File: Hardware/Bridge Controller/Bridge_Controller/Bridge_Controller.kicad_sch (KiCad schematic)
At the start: 2 parts, among them J2 AVR-UPDI-6, U2 AVR128DA64x-xPT

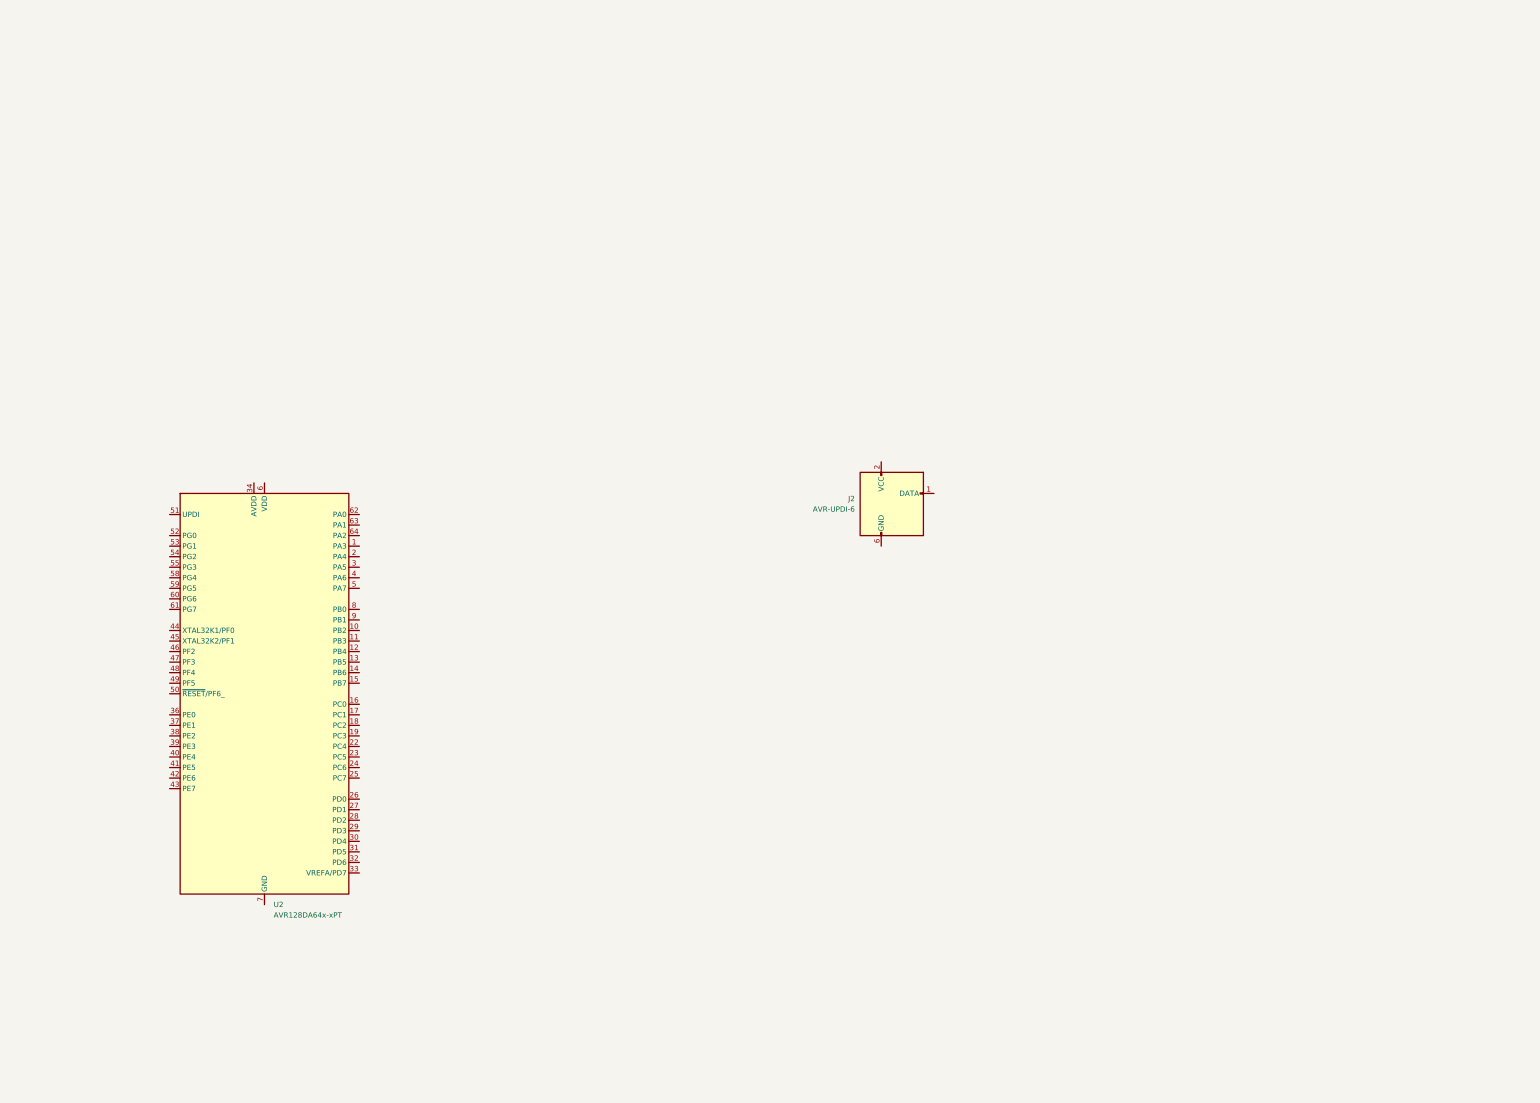
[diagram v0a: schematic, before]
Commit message: Updates to Bridge controller
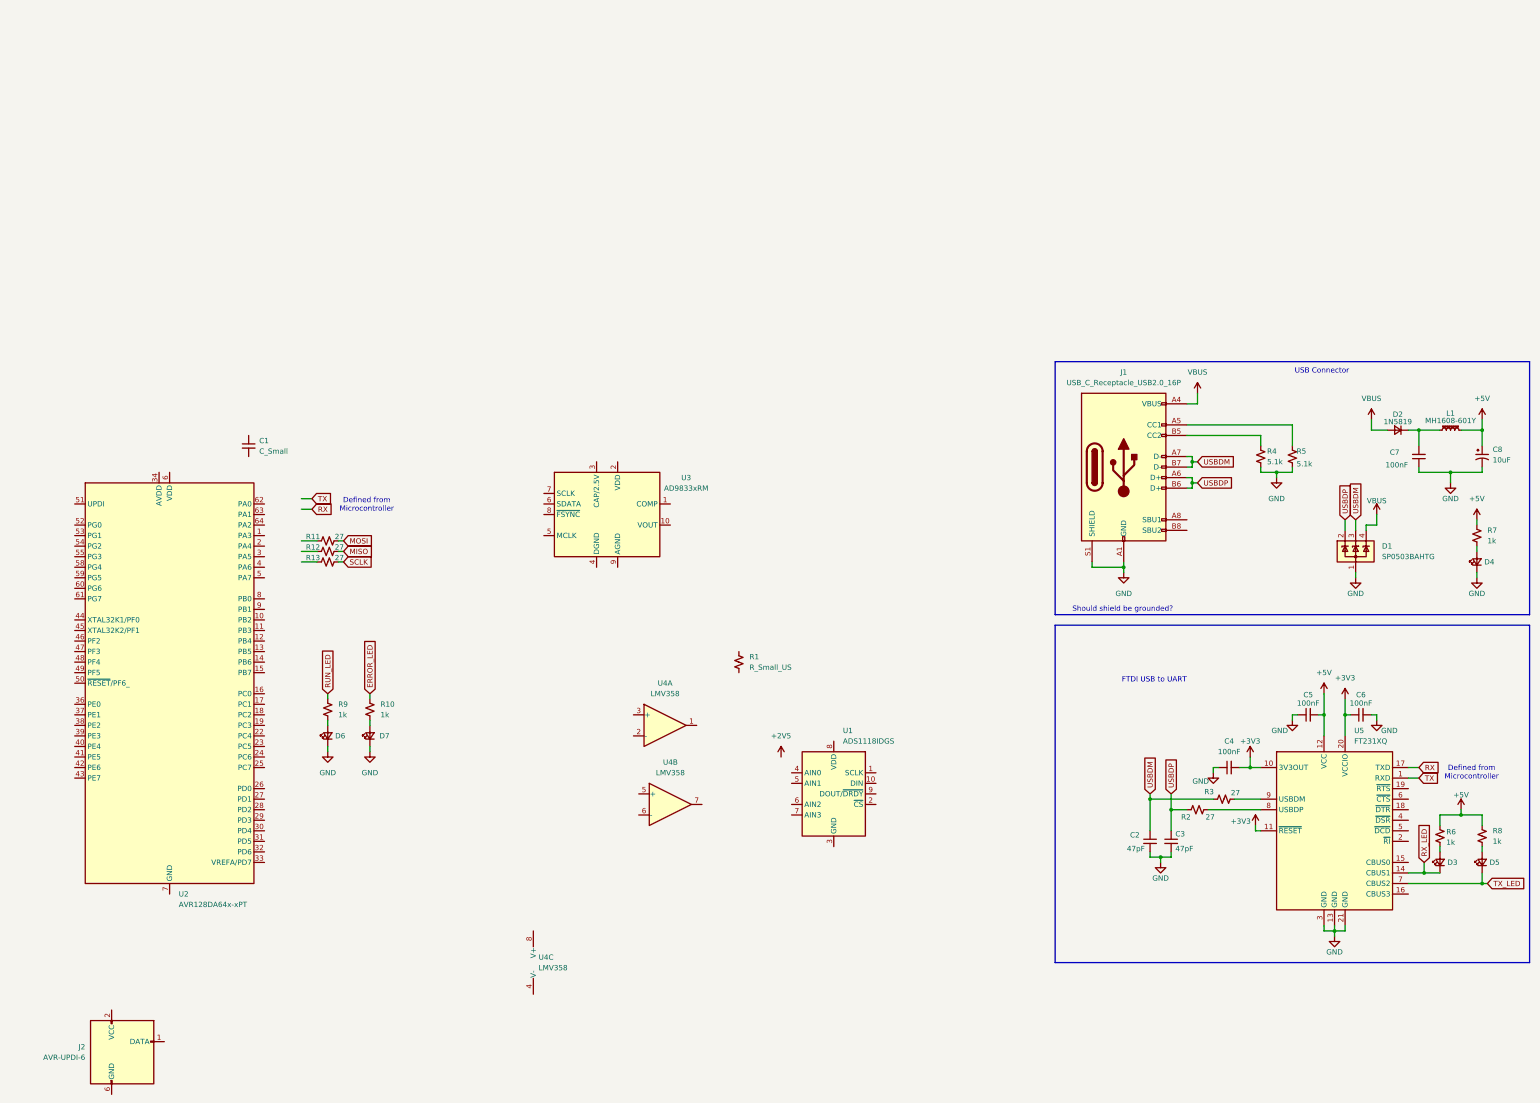
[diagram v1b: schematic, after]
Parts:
- added C1: C_Small, symbol Device:C_Small
- added C2, C3: 47pF, Capacitor_SMD:C_0402_1005Metric, symbol Device:C_Small
- added C4, C5, C6, C7: 100nF, Capacitor_SMD:C_0402_1005Metric, symbol Device:C_Small
- added C8: 10uF, Capacitor_Tantalum_SMD:CP_EIA-3216-18_Kemet-A, symbol Device:C_Polarized_Small_US
- added D1: SP0503BAHTG, Package_TO_SOT_SMD:SOT-143, symbol Power_Protection:SP0503BAHT
- added D2: 1N5819, Diode_SMD:D_SOD-123, symbol Device:D_Small
- added D3, D4, D5, D6: 150080VS75000, LED_SMD:LED_0805_2012Metric, symbol Device:LED_Small
- added D7: 150080SS75000, LED_SMD:LED_0805_2012Metric, symbol Device:LED_Small
- added J1: USB_C_Receptacle_USB2.0_16P, Connector_USB:USB_C_Receptacle_GCT_USB4085, symbol Connector:USB_C_Receptacle_USB2.0_16P
- added L1: MH1608-601Y, Inductor_SMD:L_0603_1608Metric, symbol Device:L_Ferrite_Small
- added R1: R_Small_US, symbol Device:R_Small_US
- added R10, R6, R7, R8, R9: 1k, Resistor_SMD:R_0603_1608Metric, symbol Device:R_Small_US
- added R11, R12, R13, R2, R3: 27, Resistor_SMD:R_0603_1608Metric, symbol Device:R_Small_US
- added R4, R5: 5.1k, Resistor_SMD:R_0603_1608Metric, symbol Device:R_Small_US
- added U1: ADS1118IDGS, symbol Analog_ADC:ADS1118IDGS
- added U3: AD9833xRM, Package_SO:MSOP-10_3x3mm_P0.5mm, symbol Interface:AD9833xRM
- added U4: LMV358, symbol Amplifier_Operational:LMV358
- added U5: FT231XQ, Package_DFN_QFN:QFN-20-1EP_4x4mm_P0.5mm_EP2.5x2.5mm, symbol Interface_USB:FT231XQ
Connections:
- new net: C7.2, D2.1 (K), L1.1
- new net: R2.2, U5.8 (USBDP)
- new net: R3.2, U5.9 (USBDM)
- new net: D3.2 (A), R6.2
- new net: D5.2 (A), R8.2
- new net: J1.A5 (CC1), R5.1
- new net: J1.B5 (CC2), R4.1
- new net: D4.2 (A), R7.2
- new net: D6.2 (A), R9.2
- new net: D7.2 (A), R10.2
- new net +3V3: C4.2, C6.1, U5.10 (3V3OUT), U5.11 (~{RESET}), U5.20 (VCCIO)
- new net +5V: C5.2, C8.1, L1.2, R6.1, R7.1, R8.1, U5.12 (VCC)
- new net ERROR_LED: R10.1
- new net GND: C2.2, C3.2, C4.1, C5.1, C6.2, C7.1, C8.2, D1.1 (A), D4.1 (K), D6.1 (K), D7.1 (K), J1.A1 (GND), J1.A12 (GND), J1.B1 (GND), J1.B12 (GND), J1.S1 (SHIELD), R4.2, R5.2, U5.13 (GND), U5.21 (GND), U5.3 (GND)
- new net MISO: R12.2
- new net MOSI: R11.2
- new net RUN_LED: R9.1
- new net RX: U5.17 (TXD)
- new net RX_LED: D3.1 (K), U5.14 (CBUS1)
- new net SCLK: R13.2
- new net TX: U5.1 (RXD)
- new net TX_LED: D5.1 (K), U5.7 (CBUS2)
- new net USBDM: C2.1, D1.3 (K), J1.A7 (D-), J1.B7 (D-), R3.1
- new net USBDP: C3.1, D1.2 (K), J1.A6 (D+), J1.B6 (D+), R2.1
- new net VBUS: D1.4 (K), D2.2 (A), J1.A4 (VBUS), J1.A9 (VBUS), J1.B4 (VBUS), J1.B9 (VBUS)
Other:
- note added: "Defined from Microcontroller"
- note added: "FTDI USB to UART"
- note added: "Should shield be grounded?"
- note added: "USB Connector"
- moved on the sheet: J2, U2

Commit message: Updating Bridge Controller
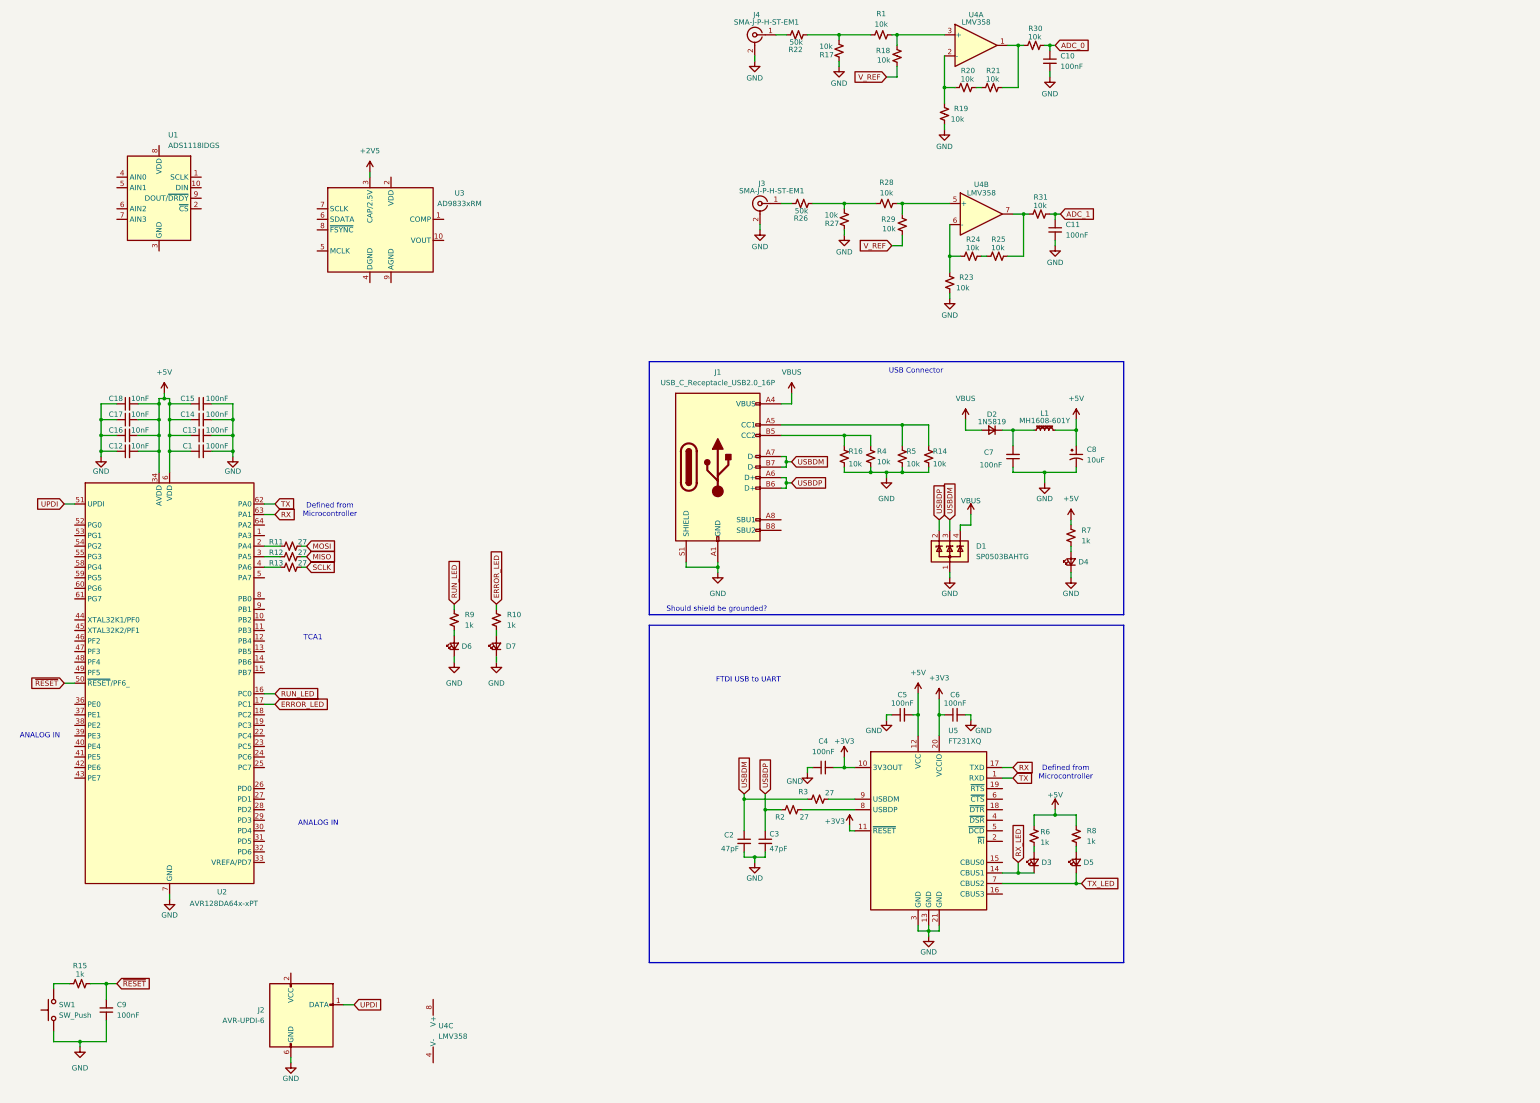
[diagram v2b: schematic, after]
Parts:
- added C10, C11, C13, C14, C15: 100nF, symbol Device:C_Small
- added C12, C16, C17, C18: 10nF, symbol Device:C_Small
- added C9: 100nF, Capacitor_SMD:C_0402_1005Metric, symbol Device:C_Small
- added J3, J4: SMA-J-P-H-ST-EM1, Connector_Coaxial:SMA_Samtec_SMA-J-P-X-ST-EM1_EdgeMount, symbol Connector:Conn_Coaxial
- added R14, R16: 10k, Resistor_SMD:R_0603_1608Metric, symbol Device:R_Small_US
- added R15: 1k, Resistor_SMD:R_0603_1608Metric, symbol Device:R_Small_US
- added R17, R18, R19, R20, R21, R23, R24, R25, R27, R28, R29, R30, R31: 10k, symbol Device:R_Small_US
- added R22, R26: 50k, symbol Device:R_Small_US
- added SW1: SW_Push, Button_Switch_SMD:SW_SPST_B3SL-1002P, symbol Switch:SW_Push
- C1: value C_Small -> 100nF
- R1: value R_Small_US -> 10k
- R4, R5: value 5.1k -> 10k
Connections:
- net +2V5: now also U3.3 (CAP/2.5V)
- net +5V: now also C1.1, U2.20 (VDD), U2.34 (AVDD), U2.56 (VDD), U2.6 (VDD), C12.2, C13.1, C14.1, C15.1, C16.2, C17.2, C18.2
- net ERROR_LED: now also U2.17 (PC1)
- net GND: now also C1.2, J2.6 (GND), U2.21 (GND), U2.35 (GND), U2.57 (GND), U2.7 (GND), C10.2, C11.2, C12.1, C13.2, C14.2, C15.2, C16.1, C17.1, C18.1, C9.1, J3.2 (Ext), J4.2 (Ext), R14.2, R16.2, R17.2, R19.1, R23.1, R27.2, SW1.1
- net RUN_LED: now also U2.16 (PC0)
- net RX: now also U2.63 (PA1)
- net TX: now also U2.62 (PA0)
- net at J1.A5 (CC1), R5.1: now also R14.1
- net at J1.B5 (CC2), R4.1: now also R16.1
- net UPDI: now reaches J2.1 (DATA)
- net UPDI: now also U2.51 (UPDI)
- net at U4.1: now also R21.1, R30.2
- net at U4.2 (-): now also R19.2, R20.2
- net at U4.3 (+): now also R1.2, R18.2
- net at U4.5 (+): now also R28.2, R29.2
- net at U4.6 (-): now also R23.2, R24.2
- net at U4.7: now also R25.1, R31.2
- net at U2.2 (PA4): now also R11.1
- net at U2.3 (PA5): now also R12.1
- net at U2.4 (PA6): now also R13.1
- net ~{RESET}: now reaches U2.50 (~{RESET}/PF6_)
- net ~{RESET}: now also C9.2, R15.2
- net at R1.1: now also R17.1, R22.2
- new net: R15.1, SW1.2
- new net: R20.1, R21.2
- new net: R26.2, R27.1, R28.1
- new net: J3.1 (In), R26.1
- new net: J4.1 (In), R22.1
- new net: R24.1, R25.2
- new net ADC_0: C10.1, R30.1
- new net ADC_1: C11.1, R31.1
- new net V_REF: R18.1, R29.1
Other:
- note added: "ANALOG IN"
- note added: "TCA1"
- moved on the sheet: C1, C2, C3, C4, C5, C6, C7, C8, D1, D2, D3, D4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

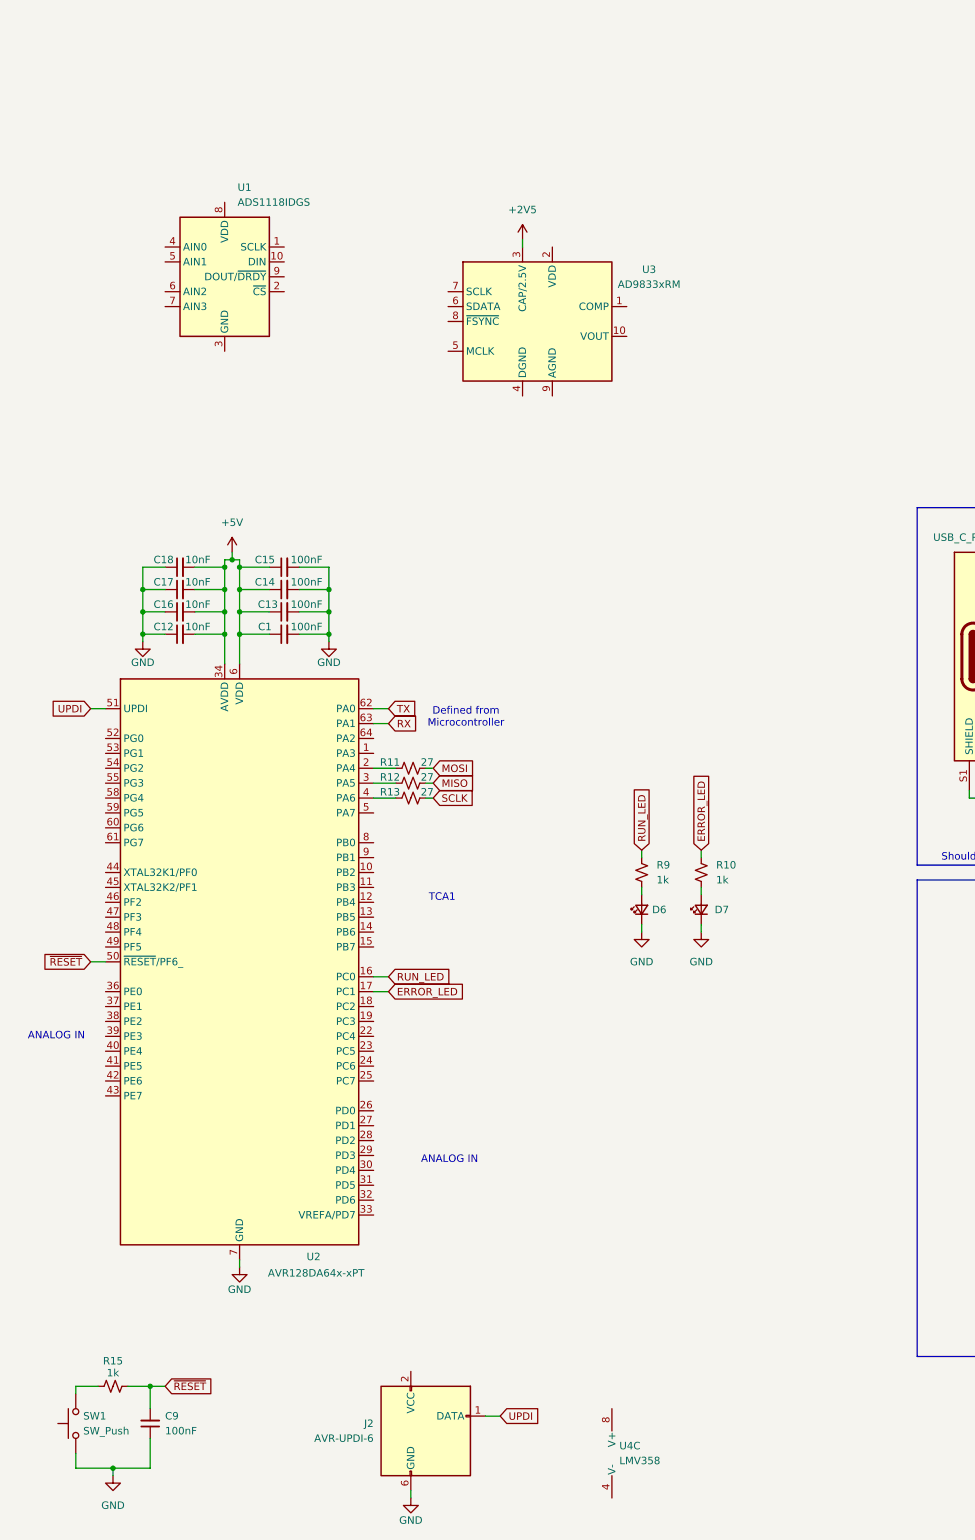
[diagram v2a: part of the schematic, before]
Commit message: Updating bridge controller
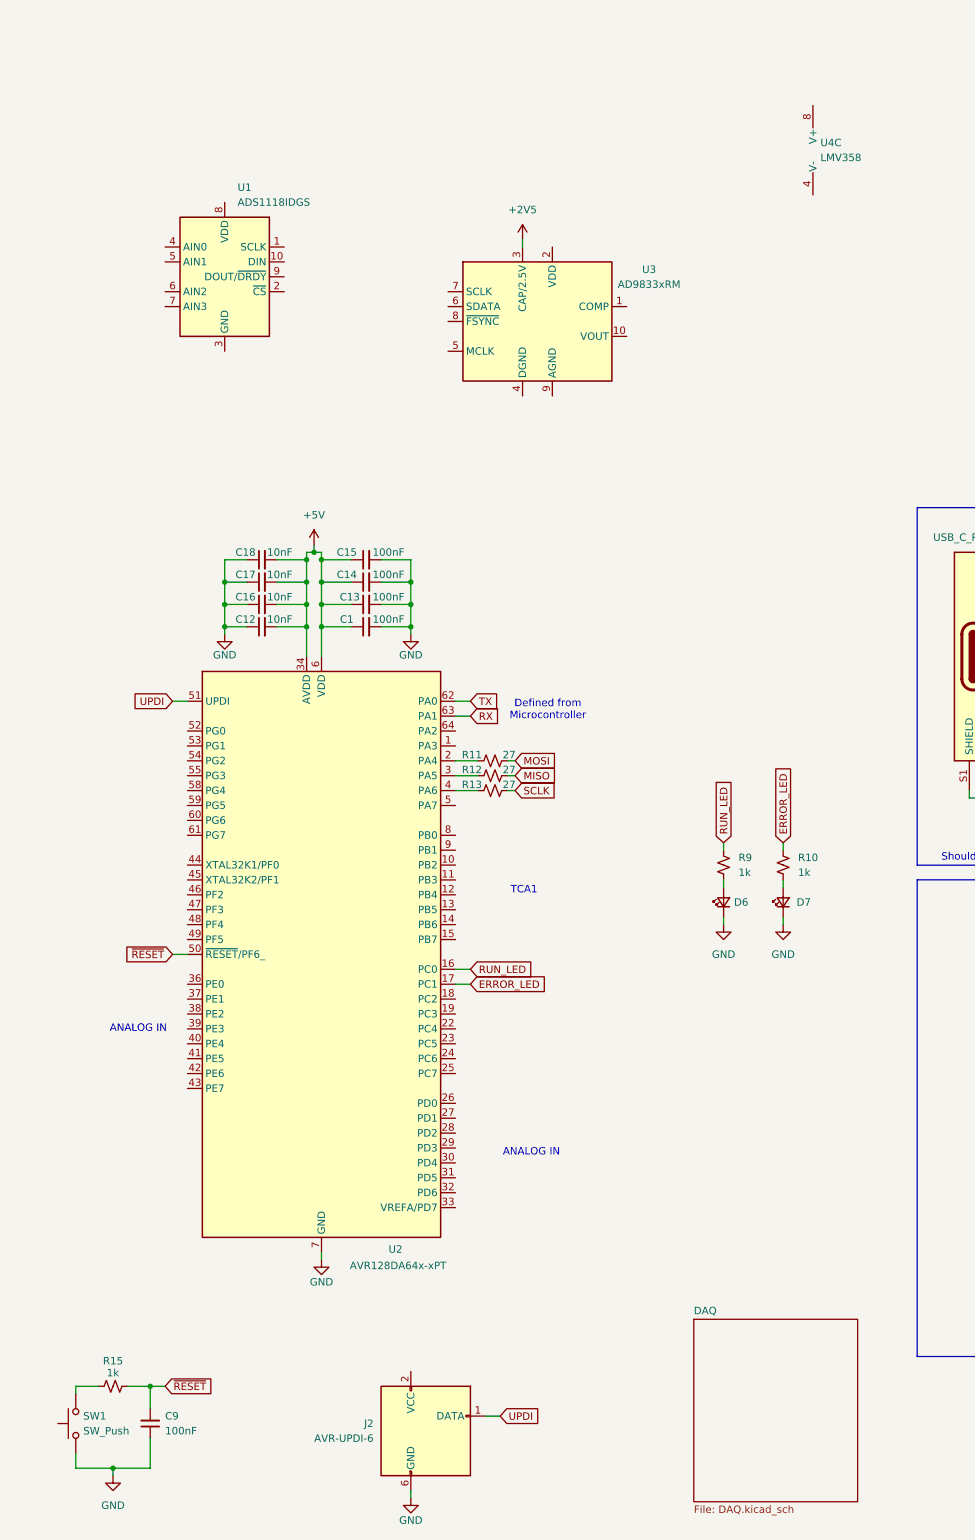
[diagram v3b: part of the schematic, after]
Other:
- added sheet DAQ (DAQ.kicad_sch)
- moved on the sheet: C1, C12, C13, C14, C15, C16, C17, C18, D6, D7, R10, R11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
